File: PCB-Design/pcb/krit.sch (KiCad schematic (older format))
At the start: 13 parts

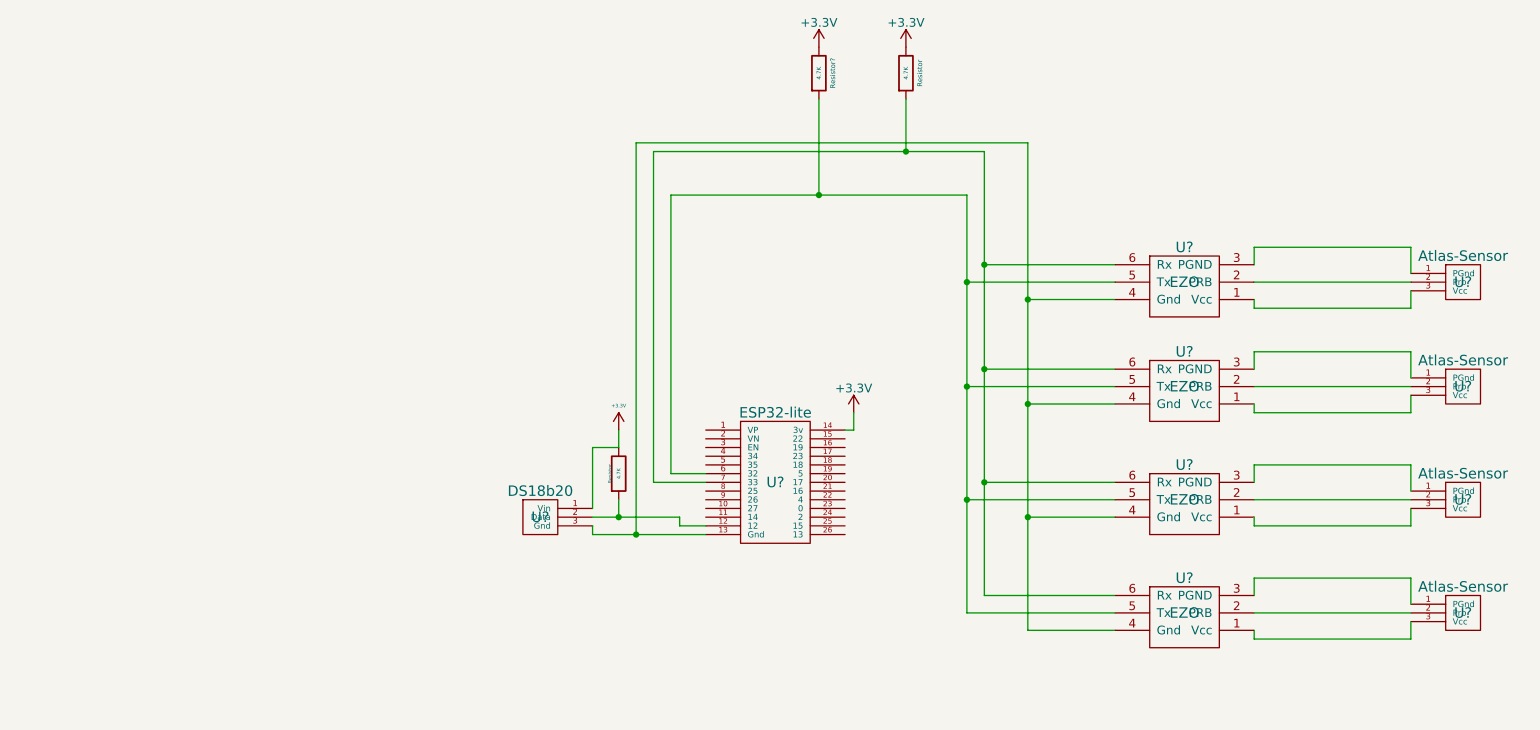
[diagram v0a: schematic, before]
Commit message: pcb complete
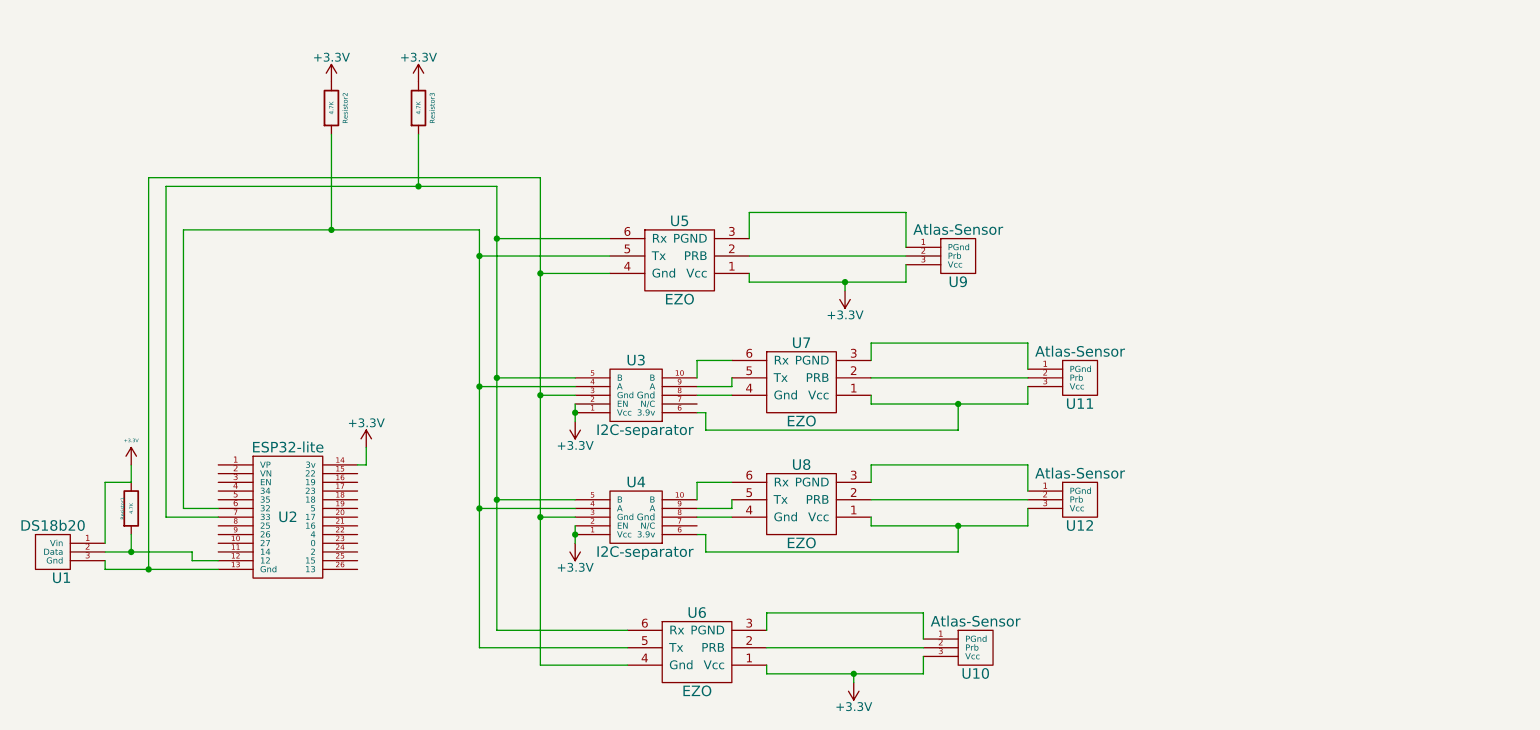
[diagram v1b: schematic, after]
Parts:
- removed U? (x2): Atlas-Sensor, symbol Atlas-Sensor
- removed U? (x2): EZO, symbol EZO
- added U11, U12: Atlas-Sensor, footprint:atlas-sensor, symbol Atlas-Sensor
- added U3, U4: I2C-separator, footprint:i2c-isolator, symbol I2C-separator
- added U7, U8: EZO, footprint:ezo, symbol EZO
- Resistor1, Resistor3: renamed from Resistor; footprint (none) -> Resistors_SMD:R_0603
- Resistor2: renamed from Resistor?; footprint (none) -> Resistors_SMD:R_0603
- U1: renamed from U?; footprint (none) -> footprint:ds18b20
- U10, U9: renamed from U?; footprint (none) -> footprint:atlas-sensor
- U2: renamed from U?; footprint (none) -> footprint:esp32-lite
- U5, U6: renamed from U?; footprint (none) -> footprint:ezo
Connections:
- net +3V3: now also U10.3 (Vcc), U5.1 (Vcc), U6.1 (Vcc), U9.3 (Vcc), U3.1 (Vcc), U3.2 (EN), U4.1 (Vcc), U4.2 (EN)
- net at U1.3 (Gnd), U2.13 (Gnd), U5.4 (Gnd)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: now also U3.3 (Gnd), U4.3 (Gnd)
- net at Resistor2.2, U2.6 (32), U5.5 (Tx)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: now also U3.4 (A), U4.4 (A)
- net at Resistor3.2, U2.7 (33), U5.6 (Rx)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: now also U3.5 (B), U4.5 (B)
- new net: U11.1 (PGnd), U7.3 (PGND)
- new net: U11.2 (Prb), U7.2 (PRB)
- new net: U11.3 (Vcc), U3.6 (3.9v), U7.1 (Vcc)
- new net: U3.8 (Gnd), U7.4 (Gnd)
- new net: U3.9 (A), U7.5 (Tx)
- new net: U3.10 (B), U7.6 (Rx)
- new net: U12.1 (PGnd), U8.3 (PGND)
- new net: U12.2 (Prb), U8.2 (PRB)
- new net: U12.3 (Vcc), U4.6 (3.9v), U8.1 (Vcc)
- new net: U4.8 (Gnd), U8.4 (Gnd)
- new net: U4.9 (A), U8.5 (Tx)
- new net: U4.10 (B), U8.6 (Rx)
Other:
- moved on the sheet: Resistor1, Resistor2, Resistor3, U1, U10, U2, U5, U6, U9
